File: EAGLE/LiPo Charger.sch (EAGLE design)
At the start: 51 parts, among them Q1 SI7617DN-T1-GE3, Q2 SI7617DN-T1-GE3, Q3 SIS412DN-T1-GE3, Q4 SIS412DN-T1-GE3, Q5 SI7617DN-T1-GE3, U1 BQ24616RGER

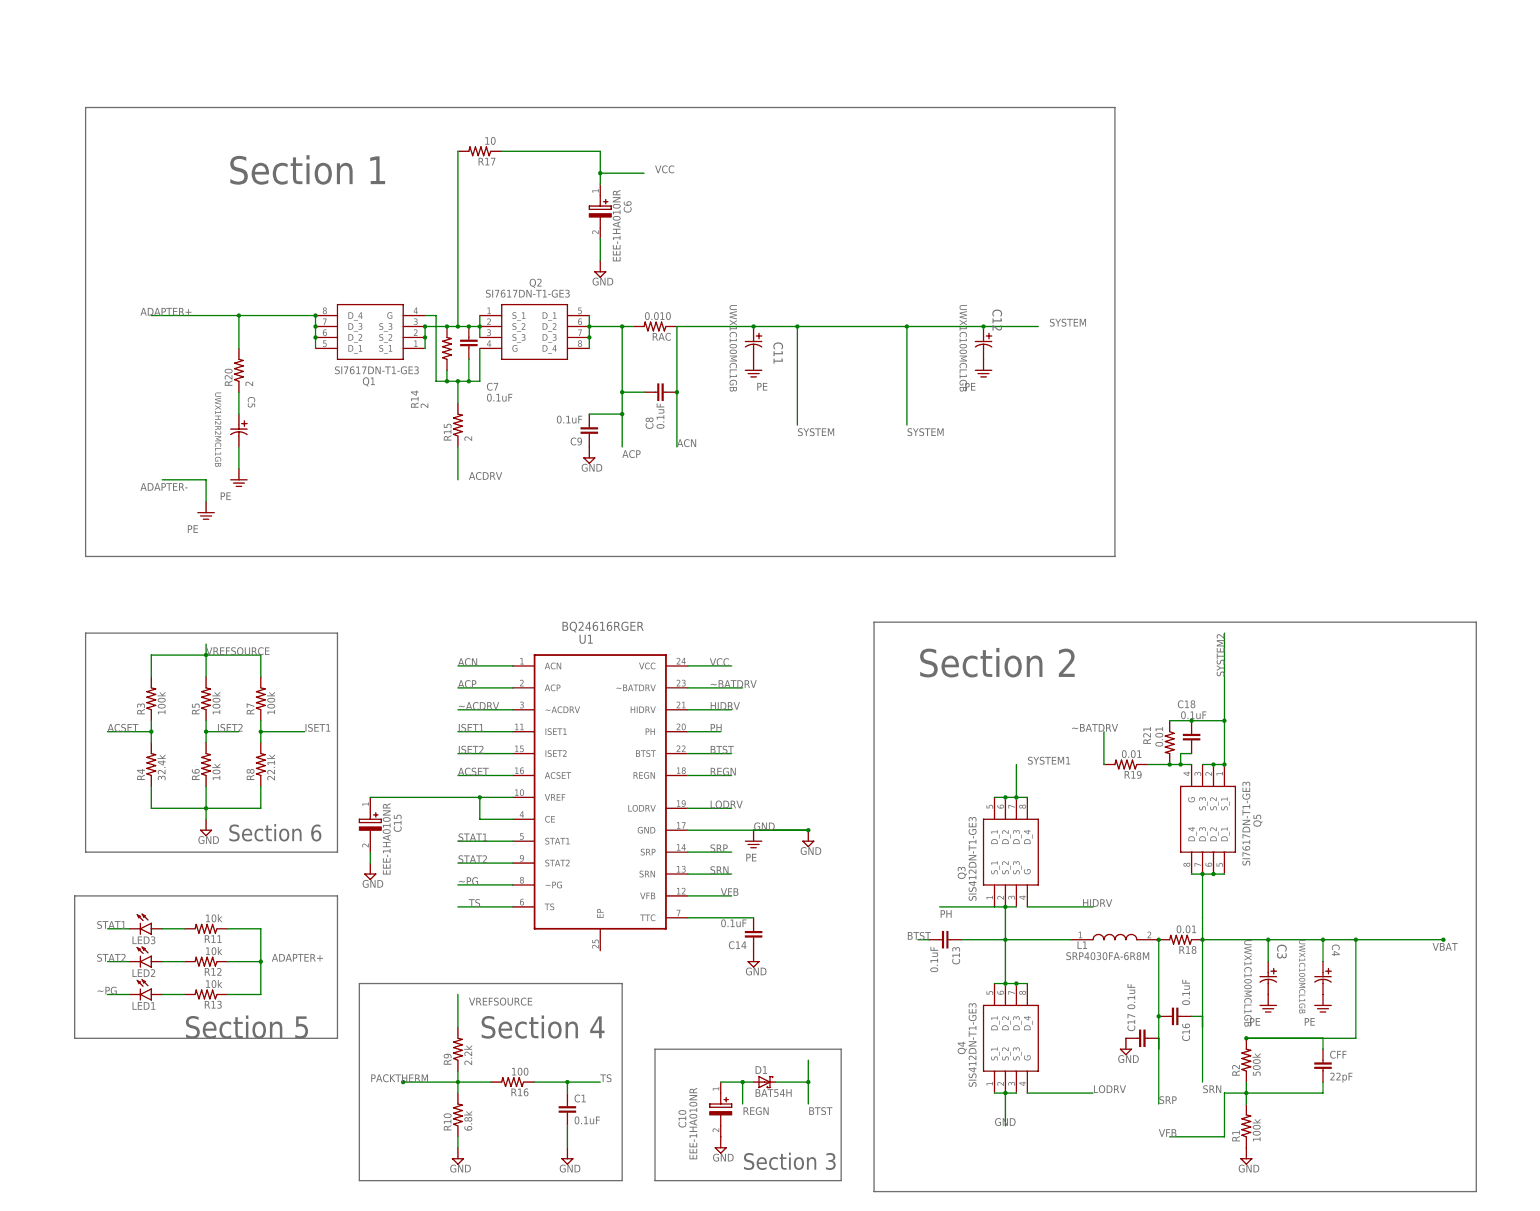
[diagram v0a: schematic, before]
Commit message: wiring f0
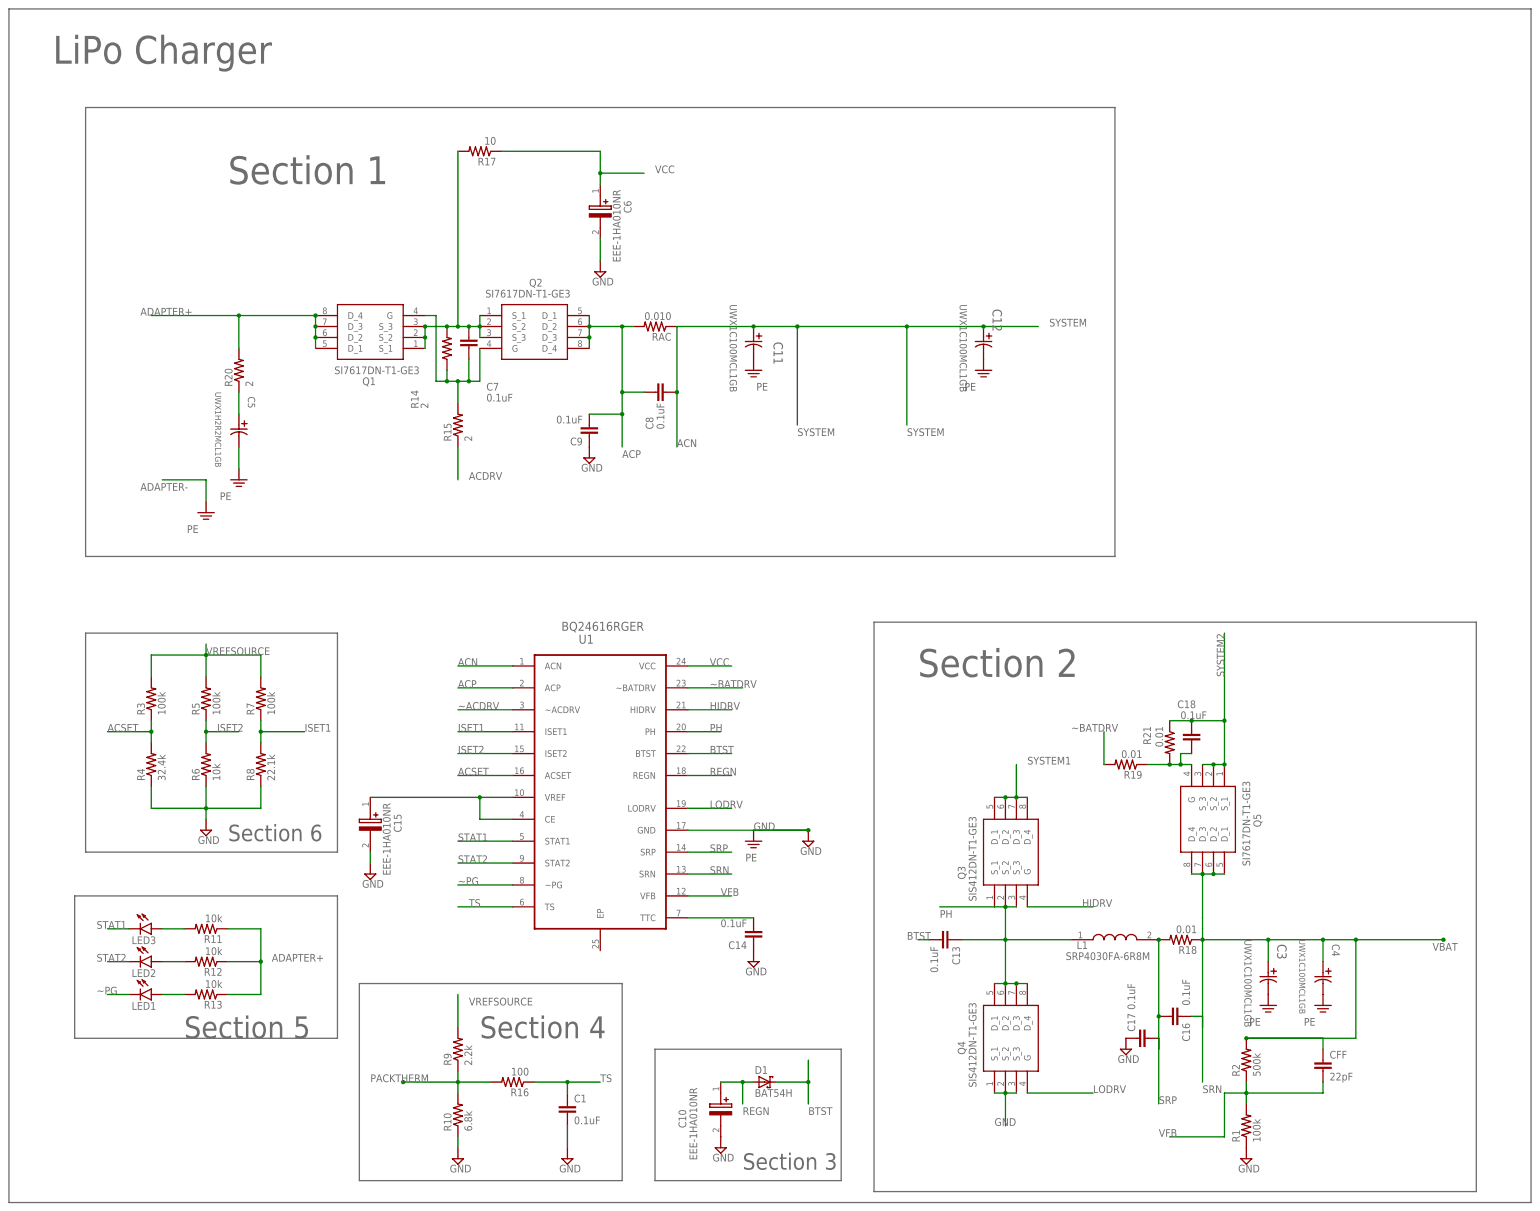
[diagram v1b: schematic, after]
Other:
- note added: "LiPo Charger"
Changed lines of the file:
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@@
 <text x="-86.36" y="-17.78" size="3.81" layer="95">Section 6</text>
 <text x="33.02" y="-93.98" size="3.81" layer="95">Section 3</text>
+<wire x1="-137.16" y1="-101.6" x2="-137.16" y2="175.26" width="0.1524" layer="95"/>
+<wire x1="-137.16" y1="175.26" x2="215.9" y2="175.26" width="0.1524" layer="95"/>
+<wire x1="215.9" y1="175.26" x2="215.9" y2="-101.6" width="0.1524" layer="95"/>
+<wire x1="215.9" y1="-101.6" x2="-137.16" y2="-101.6" width="0.1524" layer="95"/>
+<text x="-127" y="162.56" size="6.4516" layer="95">LiPo Charger</text>
 </plain>
 <instances>
